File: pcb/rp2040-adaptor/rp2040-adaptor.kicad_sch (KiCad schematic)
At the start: 3 parts, among them J1 Conn_01x09, J2 Conn_01x09

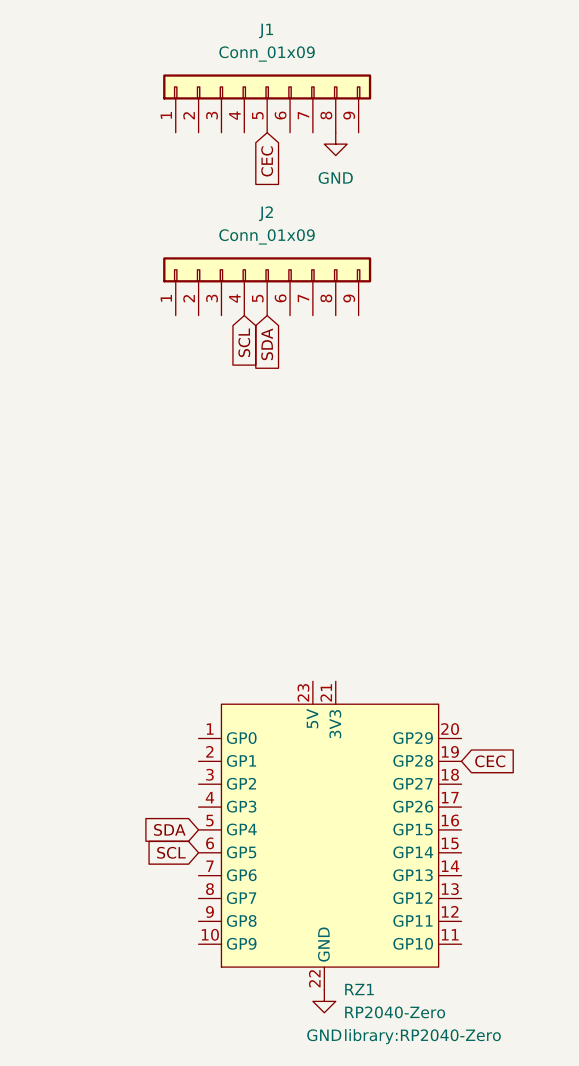
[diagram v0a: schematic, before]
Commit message: correct hardware bugs
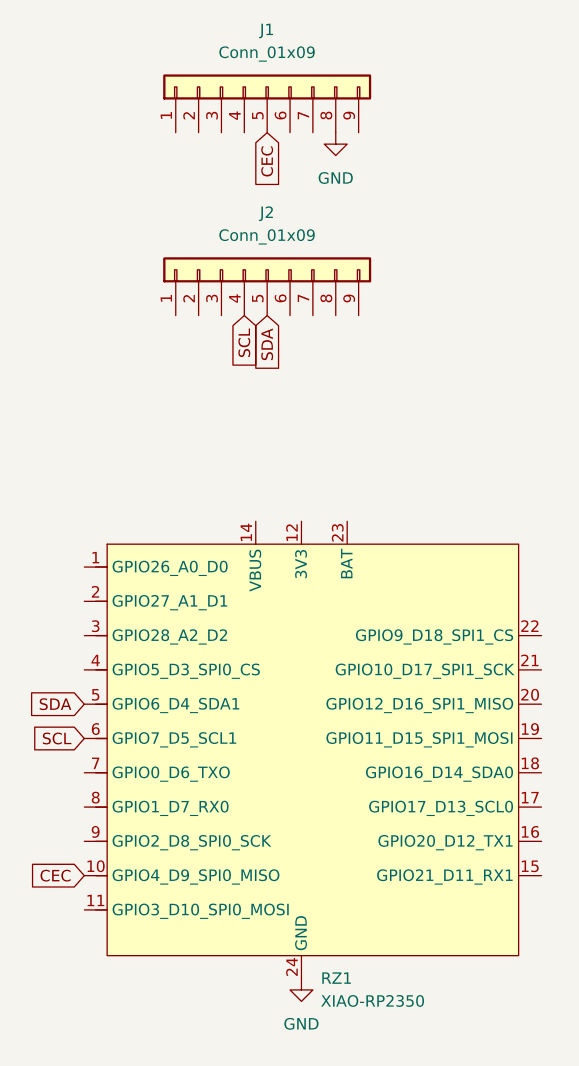
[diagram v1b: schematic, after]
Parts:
- RZ1: value RP2040-Zero -> XIAO-RP2350; footprint library:RP2040-Zero -> library:XIAO-RP2350-DIP; symbol rp2040-zero:RP2040-Zero -> Seeed_Studio_XIAO_Series:XIAO-RP2350-DIP
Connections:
- net CEC: now also RZ1.10 (GPIO4_D9_SPI0_MISO); no longer RZ1.19 (GP28)
- net GND: now also RZ1.13 (GND), RZ1.24 (GND); no longer RZ1.22 (GND)
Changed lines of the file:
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@@
 	(global_label "SCL"
 		(shape input)
-		(at 106.68 128.27 180)
+		(at 93.98 115.57 180)
 		(fields_autoplaced yes)
 		(effects
@@
 		)
 		(property "Intersheetrefs" "${INTERSHEET_REFS}"
-			(at 100.8414 128.27 0)
+			(at 88.1414 115.57 0)
 			(hide yes)
 			(show_name no)
@@
 	(global_label "SDA"
 		(shape input)
-		(at 106.68 125.73 180)
+		(at 93.98 111.76 180)
 		(fields_autoplaced yes)
 		(effects
@@
 		)
 		(property "Intersheetrefs" "${INTERSHEET_REFS}"
-			(at 100.7809 125.73 0)
+			(at 88.0809 111.76 0)
 			(hide yes)
 			(show_name no)
@@
 	(global_label "CEC"
 		(shape input)
-		(at 135.89 118.11 0)
+		(at 93.98 130.81 180)
 		(fields_autoplaced yes)
 		(effects
@@
 				(size 1.27 1.27)
 			)
-			(justify left)
+			(justify right)
 		)
 		(property "Intersheetrefs" "${INTERSHEET_REFS}"
-			(at 141.91 118.11 0)
-			(hide yes)
-			(show_name no)
-			(do_not_autoplace no)
-			(effects
-				(font
-					(size 1.27 1.27)
-				)
-				(justify left)
+			(at 87.3058 130.81 0)
+			(hide yes)
+			(show_name no)
+			(do_not_autoplace no)
+			(effects
+				(font
+					(size 1.27 1.27)
+				)
+				(justify right)
 			)
 		)
@@
 	(symbol
 		(lib_id "power:GND")
-		(at 120.65 143.51 0)
+		(at 118.11 142.24 0)
 		(unit 1)
 		(body_style 1)
@@
 		(fields_autoplaced yes)
 		(property "Reference" "#PWR02"
-			(at 120.65 149.86 0)
+			(at 118.11 148.59 0)
 			(hide yes)
 			(show_name no)
@@
 		)
 		(property "Value" "GND"
-			(at 120.65 148.59 0)
+			(at 118.11 147.32 0)
 			(show_name no)
 			(do_not_autoplace no)
@@
 		)
 		(property "Footprint" ""
-			(at 120.65 143.51 0)
+			(at 118.11 142.24 0)
 			(hide yes)
 			(show_name no)
@@
 		)
 		(property "Datasheet" ""
-			(at 120.65 143.51 0)
+			(at 118.11 142.24 0)
 			(hide yes)
 			(show_name no)
@@
 		)
 		(property "Description" "Power symbol creates a global label with name \"GND\" , ground"
-			(at 120.65 143.51 0)
+			(at 118.11 142.24 0)
 			(hide yes)
 			(show_name no)
@@
 	)
 	(symbol
-		(lib_id "rp2040-zero:RP2040-Zero")
-		(at 120.65 125.73 0)
+		(lib_id "Seeed_Studio_XIAO_Series:XIAO-RP2350-DIP")
+		(at 118.11 119.38 0)
 		(unit 1)
 		(body_style 1)
@@
 		(fields_autoplaced yes)
 		(property "Reference" "RZ1"
-			(at 122.7933 143.51 0)
+			(at 120.2533 142.24 0)
 			(show_name no)
 			(do_not_autoplace no)
@@
 			)
 		)
-		(property "Value" "RP2040-Zero"
-			(at 122.7933 146.05 0)
+		(property "Value" "XIAO-RP2350"
+			(at 120.2533 144.78 0)
 			(show_name no)
 			(do_not_autoplace no)
@@
 			)
 		)
-		(property "Footprint" "library:RP2040-Zero"
-			(at 122.7933 148.59 0)
-			(show_name no)
-			(do_not_autoplace no)
-			(effects
-				(font
-					(size 1.27 1.27)
-				)
-				(justify left)
+		(property "Footprint" "library:XIAO-RP2350-DIP"
+			(at 118.364 141.478 0)
+			(hide yes)
+			(show_name no)
+			(do_not_autoplace no)
+			(effects
+				(font
+					(size 1.27 1.27)
+				)
 			)
 		)
 		(property "Datasheet" ""
-			(at 120.65 125.73 0)
+			(at 118.11 107.95 0)
 			(hide yes)
 			(show_name no)
@@
 		)
 		(property "Description" ""
-			(at 120.65 125.73 0)
+			(at 118.11 107.95 0)
 			(hide yes)
 			(show_name no)
@@
 		(pin "9"
 		)
+		(pin "24"
+		)
 		(instances
